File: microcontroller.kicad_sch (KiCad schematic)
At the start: 1 part, among them U901 STM32F103RBTx

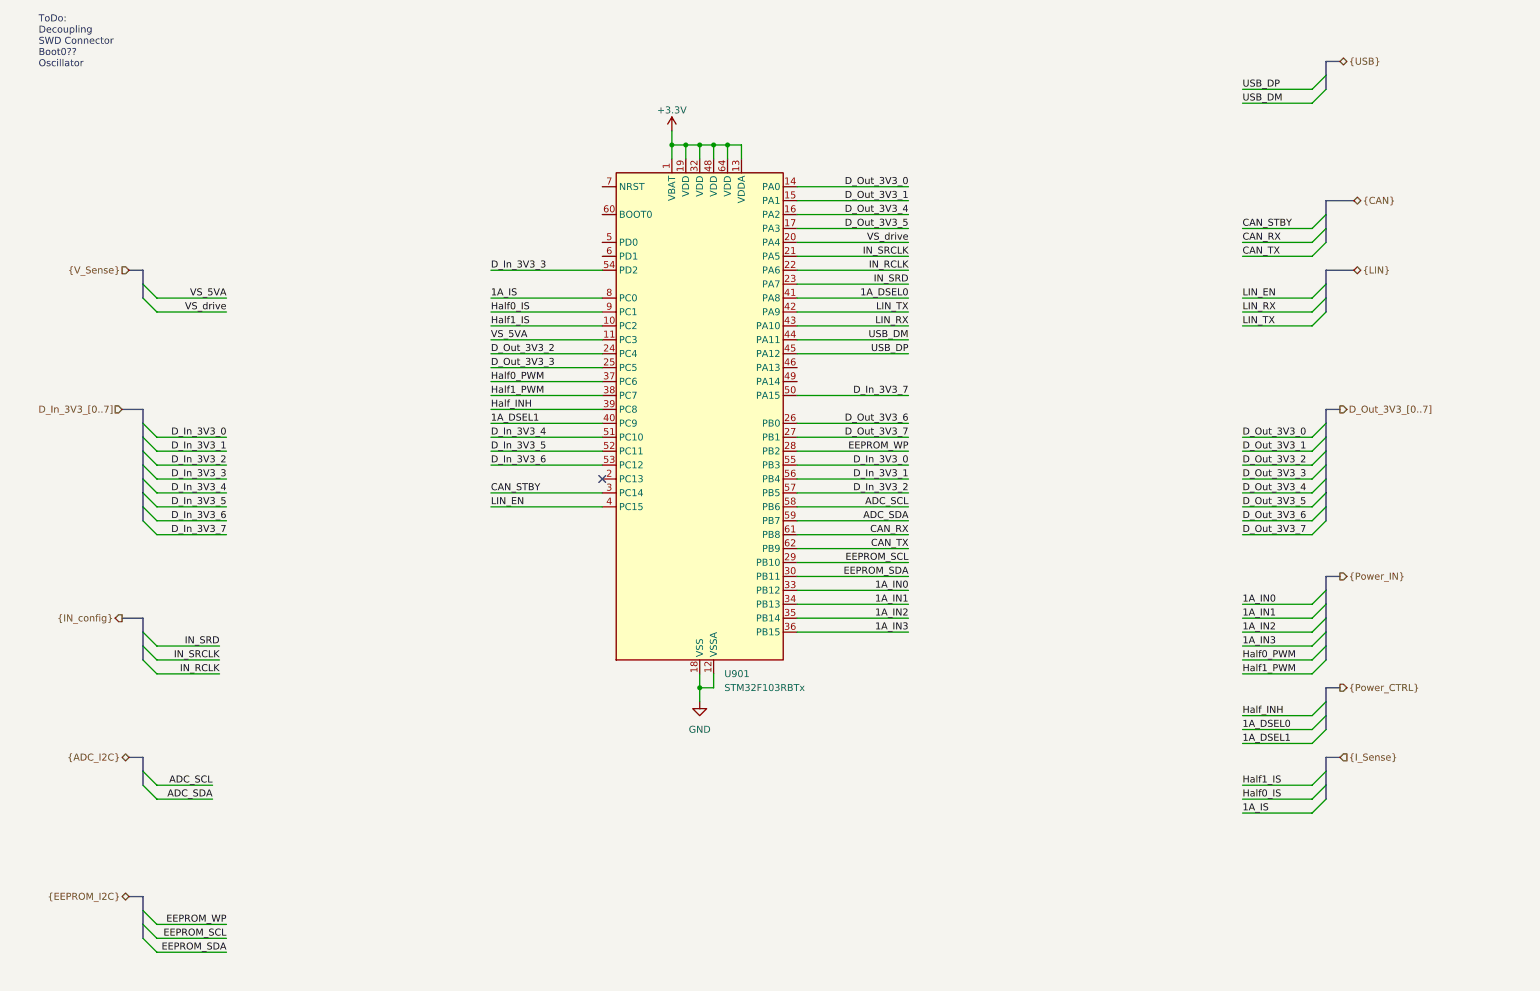
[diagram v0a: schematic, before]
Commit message: completed schematic
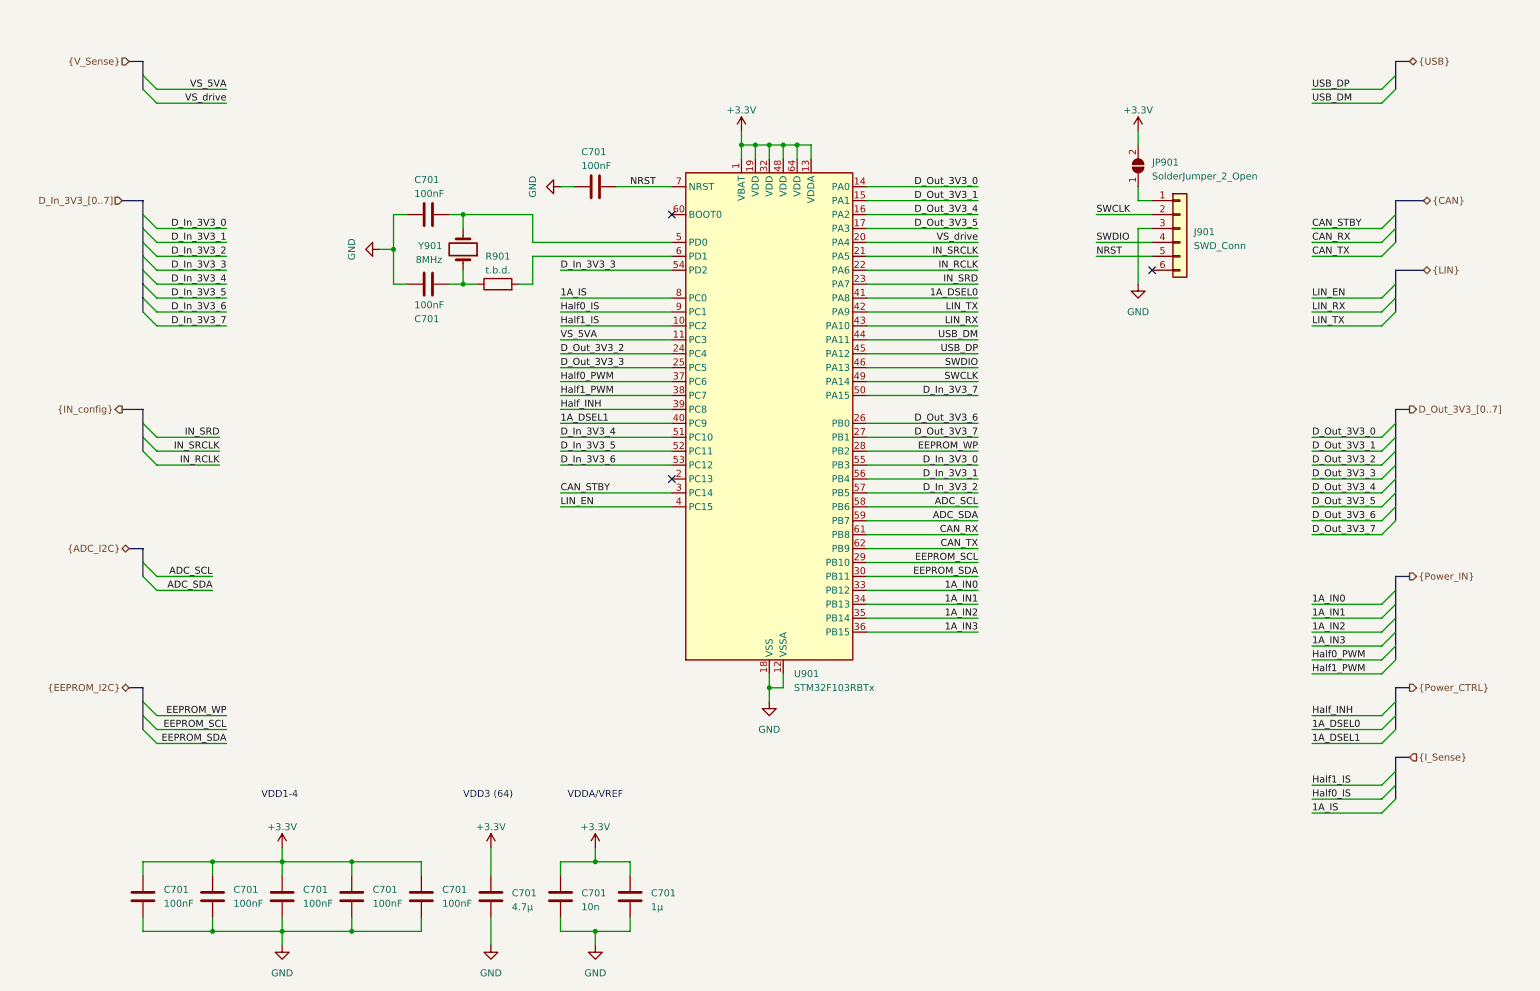
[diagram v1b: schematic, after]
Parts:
- added C701 (x8): 100nF, Capacitor_SMD:C_0603_1608Metric, symbol Device:C
- added C701: 1µ, Capacitor_SMD:C_0603_1608Metric, symbol Device:C
- added C701: 10n, Capacitor_SMD:C_0603_1608Metric, symbol Device:C
- added C701: 4.7µ, Capacitor_SMD:C_0603_1608Metric, symbol Device:C
- added J901: SWD_Conn, Connector_PinHeader_2.54mm:PinHeader_1x06_P2.54mm_Vertical, symbol Connector_Generic:Conn_01x06
- added JP901: SolderJumper_2_Open, Jumper:SolderJumper-2_P1.3mm_Open_Pad1.0x1.5mm, symbol Jumper:SolderJumper_2_Open
- added R901: t.b.d., Resistor_SMD:R_0603_1608Metric, symbol Device:R
- added Y901: 8MHz, Crystal:Crystal_SMD_3225-4Pin_3.2x2.5mm, symbol Device:Crystal
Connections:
- net +3.3V: now also C701.1, C701.1, C701.1, C701.1, C701.1, C701.1, C701.1, C701.1, JP901.2 (B)
- net GND: now also C701.2, C701.2, C701.2, C701.2, C701.2, C701.2, C701.2, C701.2, C701.2, C701.2, C701.2, J901.3 (Pin_3)
- net SWDIO: now reaches U901.46 (PA13)
- net SWDIO: now also J901.4 (Pin_4)
- net SWCLK: now reaches U901.49 (PA14)
- net SWCLK: now also J901.2 (Pin_2)
- net at U901.5 (PD0): now also C701.1, Y901.2
- net at U901.6 (PD1): now also R901.2
- net NRST: now reaches U901.7 (NRST)
- net NRST: now also C701.1, J901.5 (Pin_5)
- new net: C701.1, R901.1, Y901.1
- new net: J901.1 (Pin_1), JP901.1 (A)
- no-connect marks 1 -> 3
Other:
- note added: "VDD1-4"
- note added: "VDD3 (64)"
- note added: "VDDA/VREF"
- note removed: "ToDo: Decoupling SWD Connector Boot0?? Oscillator"
- moved on the sheet: U901
